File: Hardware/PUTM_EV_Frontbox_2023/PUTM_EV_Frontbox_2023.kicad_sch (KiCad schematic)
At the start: 29 parts, among them J2 Conn_01x04, J5 Conn_02x14_Counter_Clockwise, SW1 Reset switch, U1 STM32G473RCTx

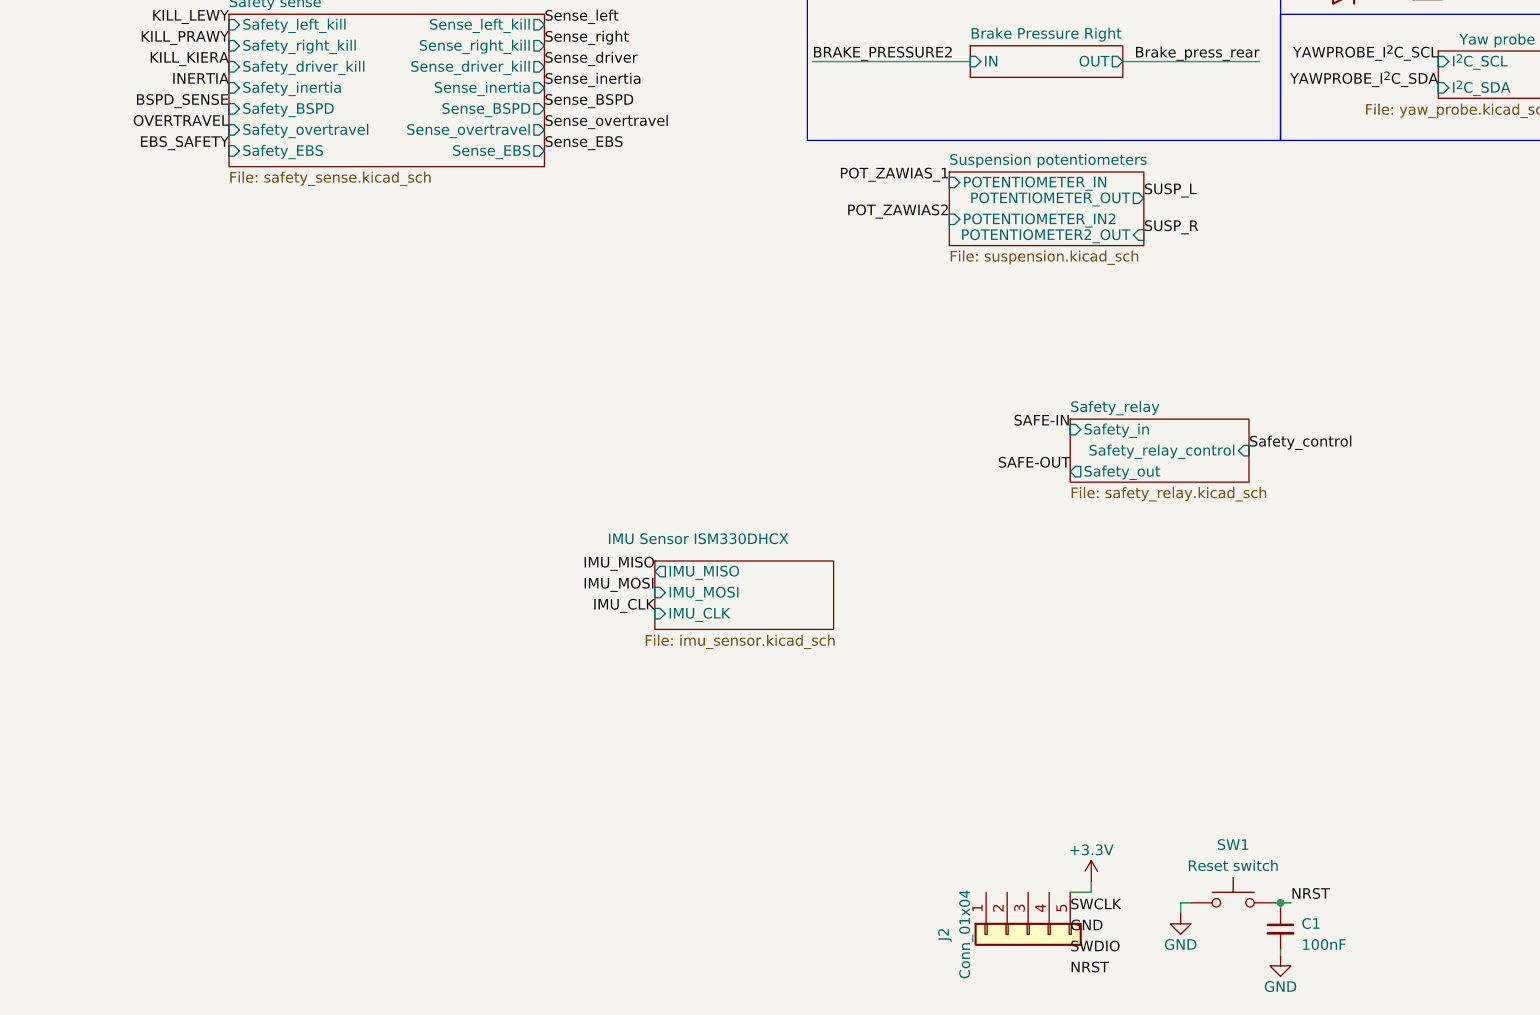
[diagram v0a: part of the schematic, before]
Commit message: Merged branch new_apps
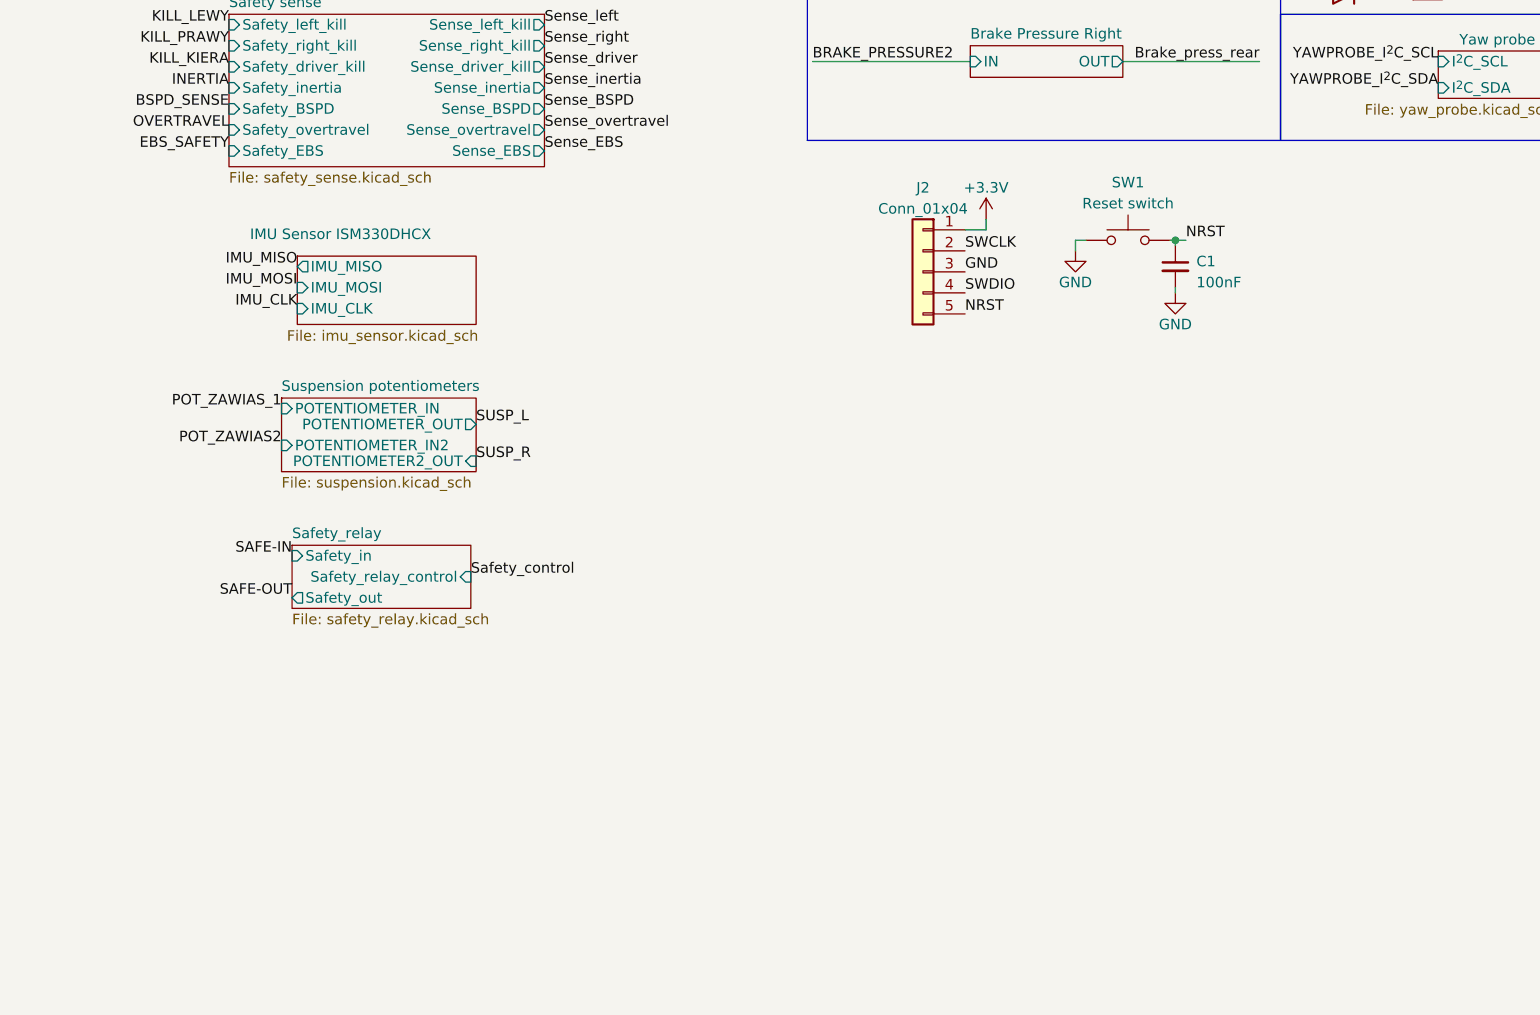
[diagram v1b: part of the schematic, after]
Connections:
- net +3.3V: now also J2.1 (Pin_1); no longer J2.5 (Pin_5)
- net GND: now also J2.3 (Pin_3)
- net NRST: now also J2.5 (Pin_5)
- net SWCLK: now also J2.2 (Pin_2)
- net SWDIO: now also J2.4 (Pin_4)
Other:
- moved on the sheet: C1, J2, SW1
